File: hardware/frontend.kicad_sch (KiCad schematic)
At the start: 113 parts, among them J1 Conn_01x12, J5001 EXT_NTC, J5002 EXT_NTC, J5003 Conn_01x07, J5004 Conn_01x03, J5005 Conn_01x11, J5006 BAT-, J5007 PACK-, Q5001 IPT015N10N5, Q5002 IPT015N10N5, U5002 BQ769x2, U5003 BQ769x2

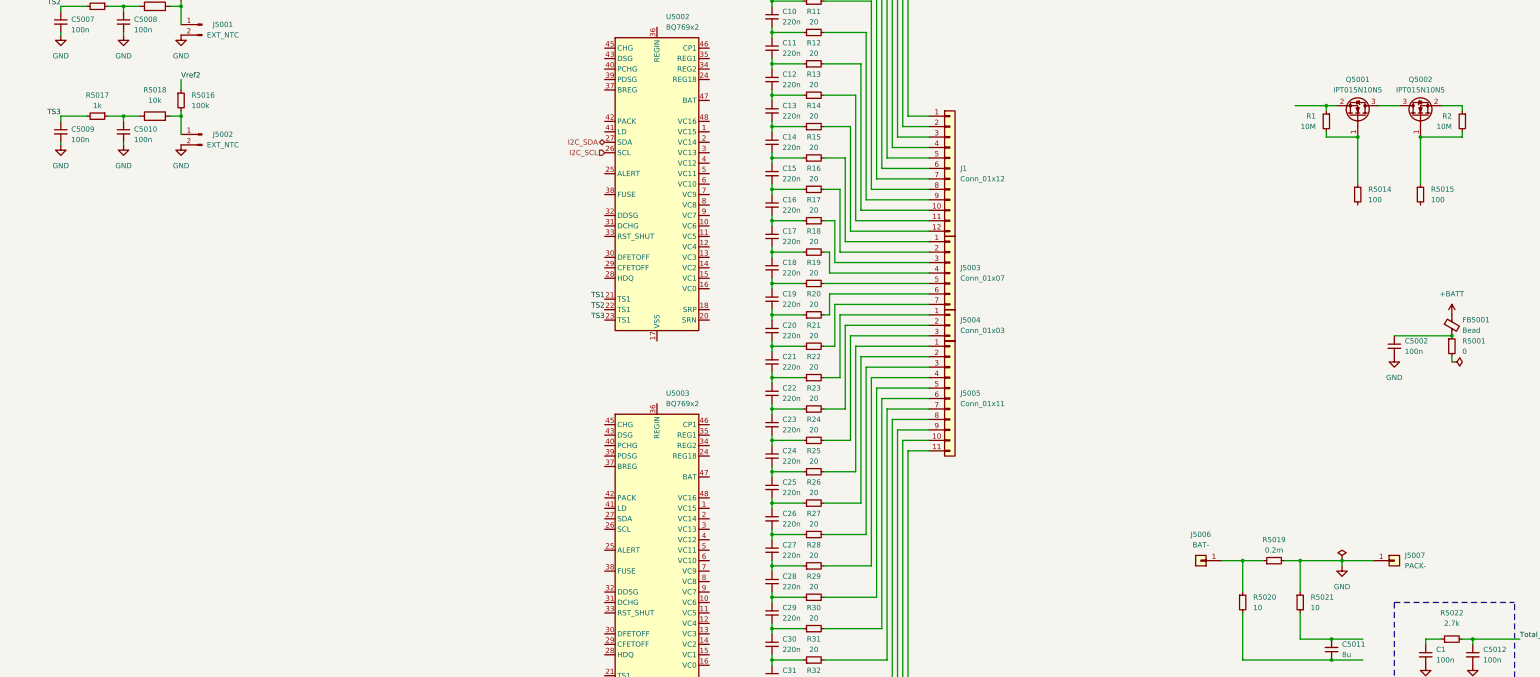
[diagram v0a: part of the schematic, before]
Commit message: Add low-side switching circuitry
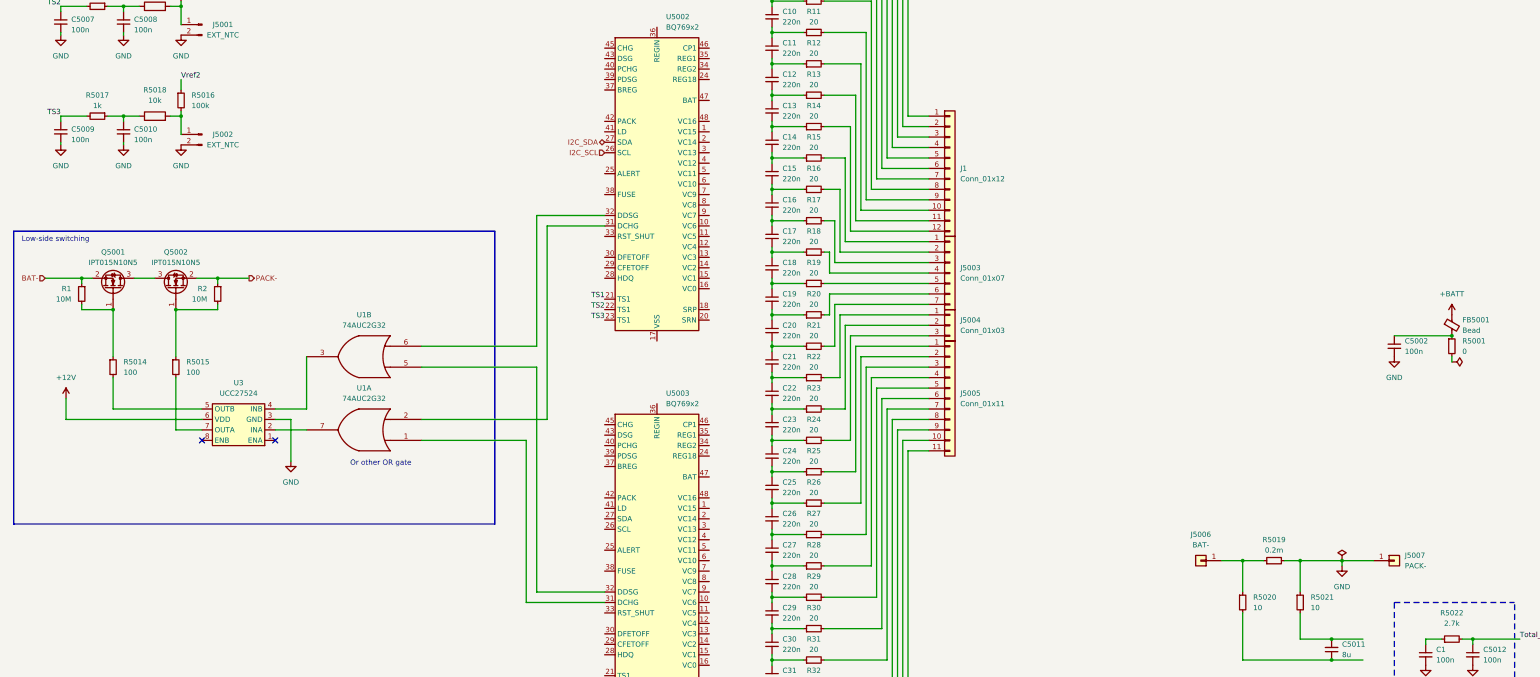
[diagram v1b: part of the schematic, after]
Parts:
- added U1: 74AUC2G32, symbol 74xGxx:74AUC2G32
- added U3: UCC27524, symbol greenmobi-bms:UCC27524
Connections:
- net GND: now also U3.3 (GND)
- net BAT-: now reaches Q5001.2 (S), R1.1
- net PACK-: now reaches Q5002.2 (S), R2.1
- net at R5015.2: now also U3.7 (OUTA)
- net at R5014.2: now also U3.5 (OUTB)
- net at U5003.31 (DCHG): now also U1.1
- net at U5003.32 (DDSG): now also U1.5
- net at U5002.31 (DCHG): now also U1.2
- net at U5002.32 (DDSG): now also U1.6
- new net: U1.7, U3.2 (INA)
- new net: U1.3, U3.4 (INB)
- new net +12V: U3.6 (VDD)
- no-connect marks 0 -> 2
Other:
- note added: "Low-side switching"
- note added: "Or other OR gate"
- moved on the sheet: Q5001, Q5002, R1, R2, R5014, R5015
